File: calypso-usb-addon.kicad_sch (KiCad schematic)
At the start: 11 parts, among them J1 Conn_02x12_Odd_Even, J2 Conn_02x12_Odd_Even, J3 USB_B_Micro, J4 USB_A_Stacked, J5 USB_A_Stacked, U1 HS8836A

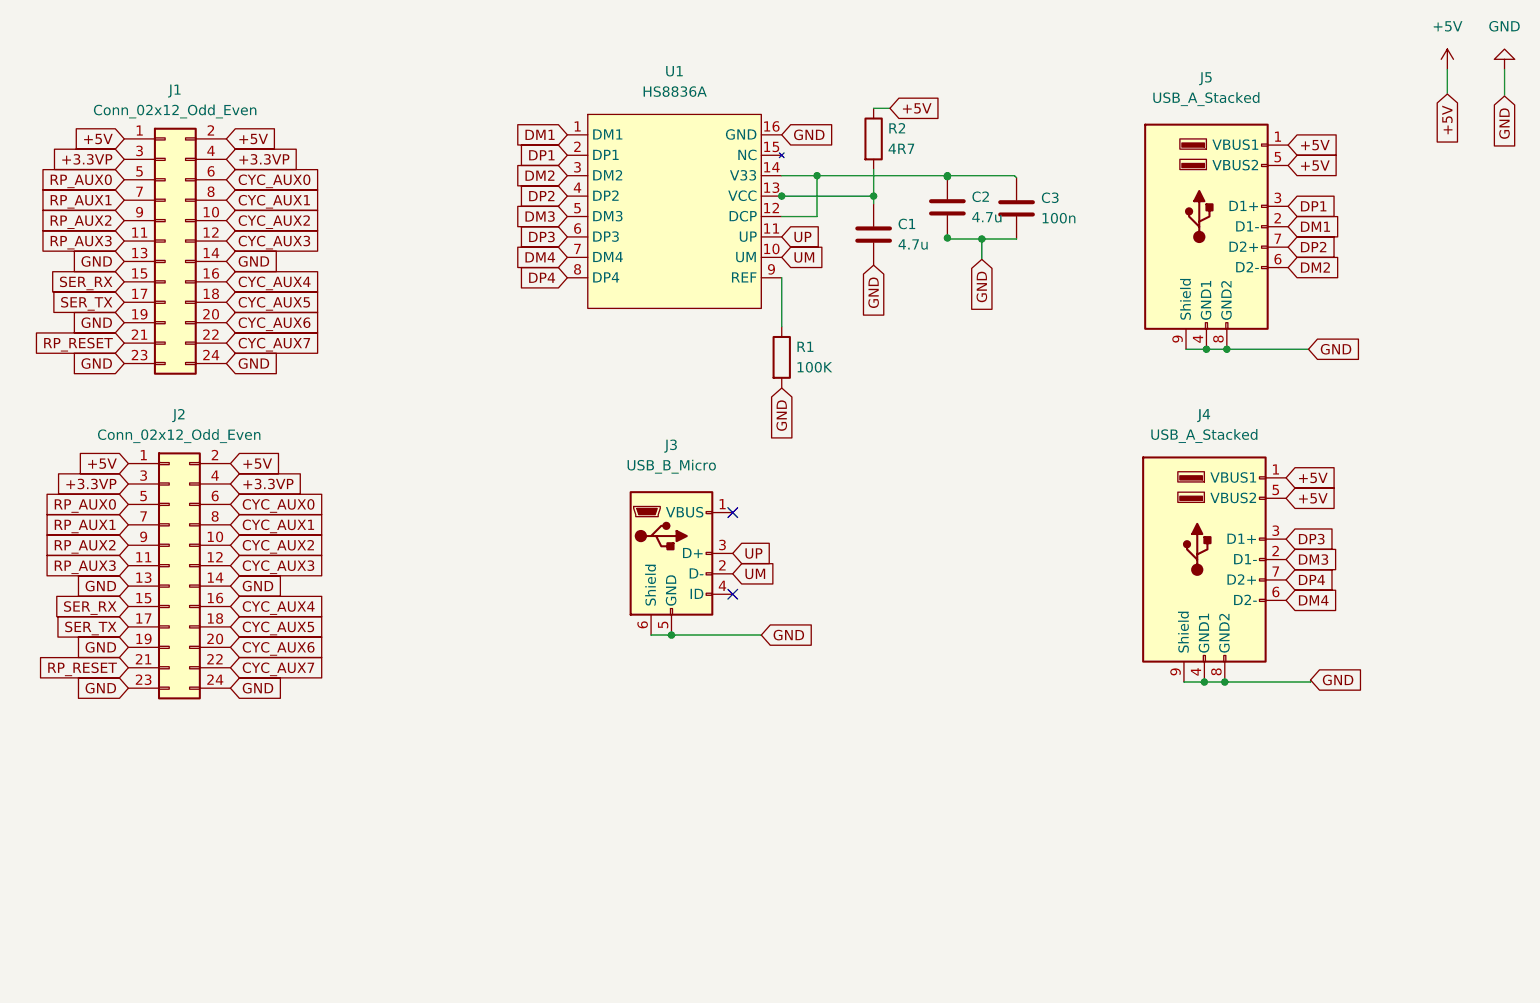
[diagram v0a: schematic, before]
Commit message: psram addition
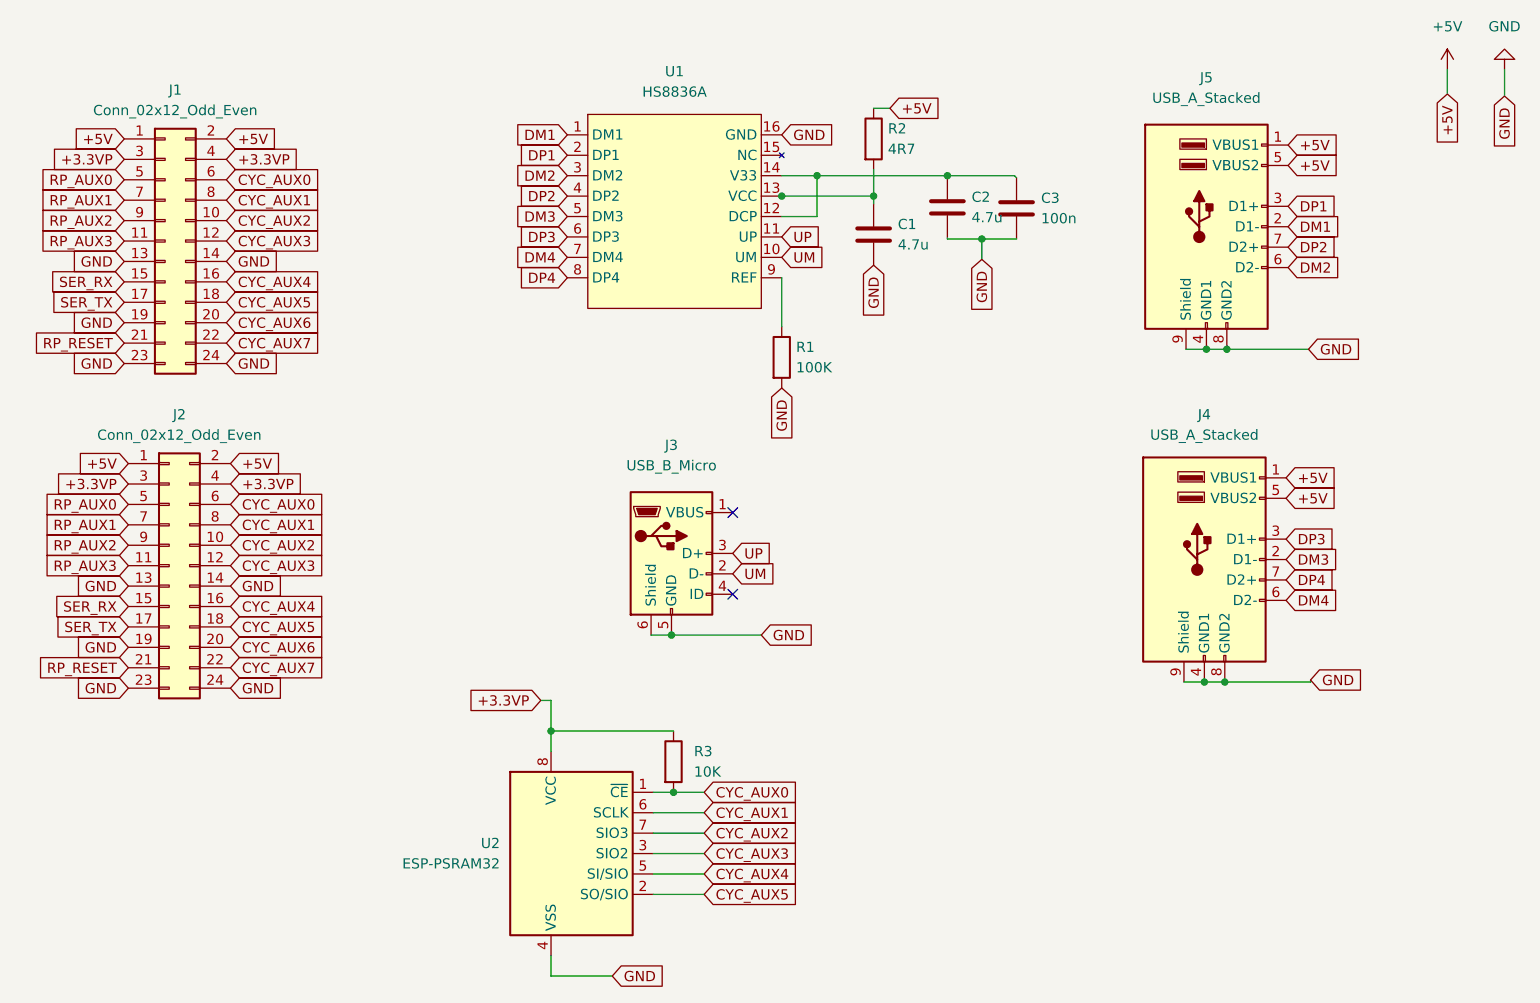
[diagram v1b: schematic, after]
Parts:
- added R3: 10K, Resistor_SMD:R_1206_3216Metric_Pad1.30x1.75mm_HandSolder, symbol Device:R
- added U2: ESP-PSRAM32, Package_SO:SOIC-8_3.9x4.9mm_P1.27mm, symbol Memory_RAM:ESP-PSRAM32
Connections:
- net +3.3VP: now also R3.1, U2.8 (VCC)
- net CYC_AUX0: now also R3.2, U2.1 (~{CE})
- net CYC_AUX1: now also U2.6 (SCLK)
- net CYC_AUX2: now also U2.7 (SIO3)
- net CYC_AUX3: now also U2.3 (SIO2)
- net CYC_AUX4: now also U2.5 (SI/SIO)
- net CYC_AUX5: now also U2.2 (SO/SIO)
- net GND: now also U2.4 (VSS)
